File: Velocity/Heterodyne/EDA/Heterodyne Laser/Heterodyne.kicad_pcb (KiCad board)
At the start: 2 copper layers, 35.5 x 19 mm, 38 parts, among them J1 Conn_01x05, J7 Reciever, U1 SA612AD, U2 NE5532DR, U3 MAX7375AXR105, U4 MAX11613, U5 ATmega328PB-AU, Y1 8 MHz

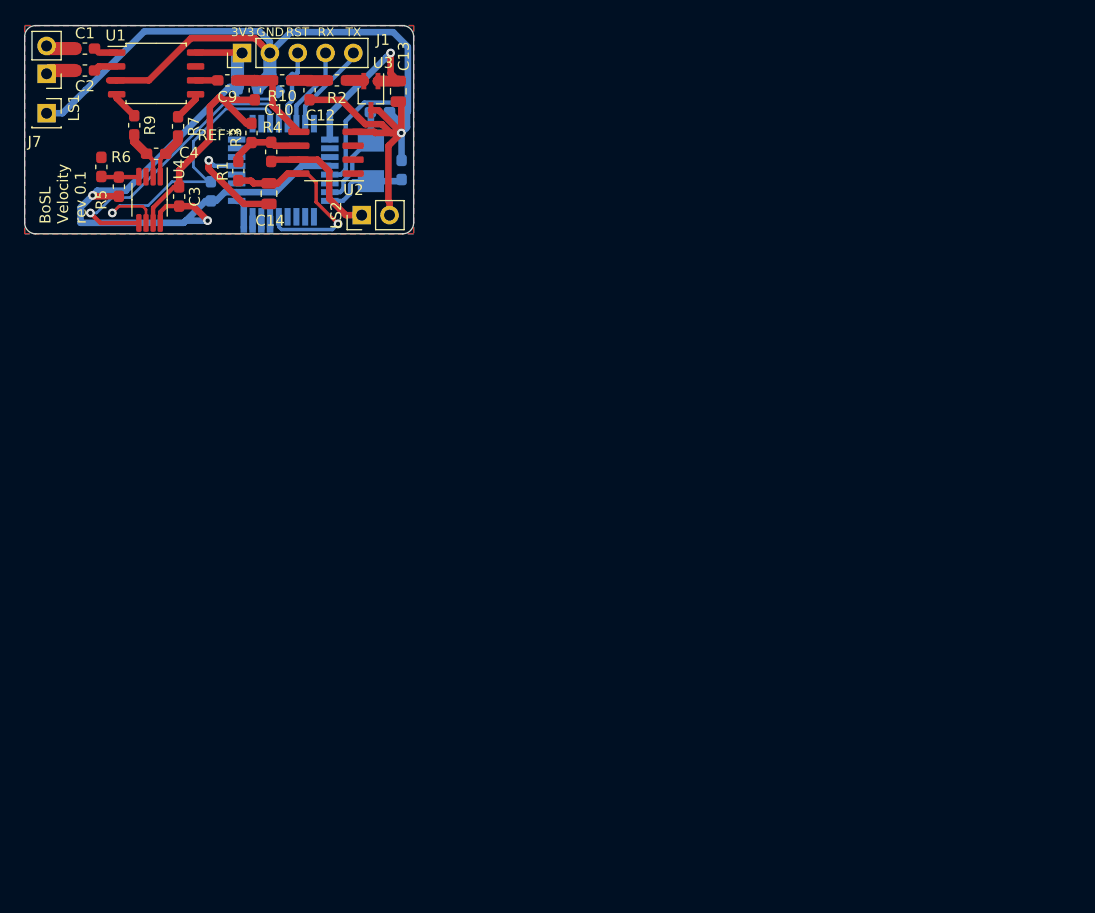
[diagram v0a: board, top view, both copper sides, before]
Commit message: daily commit
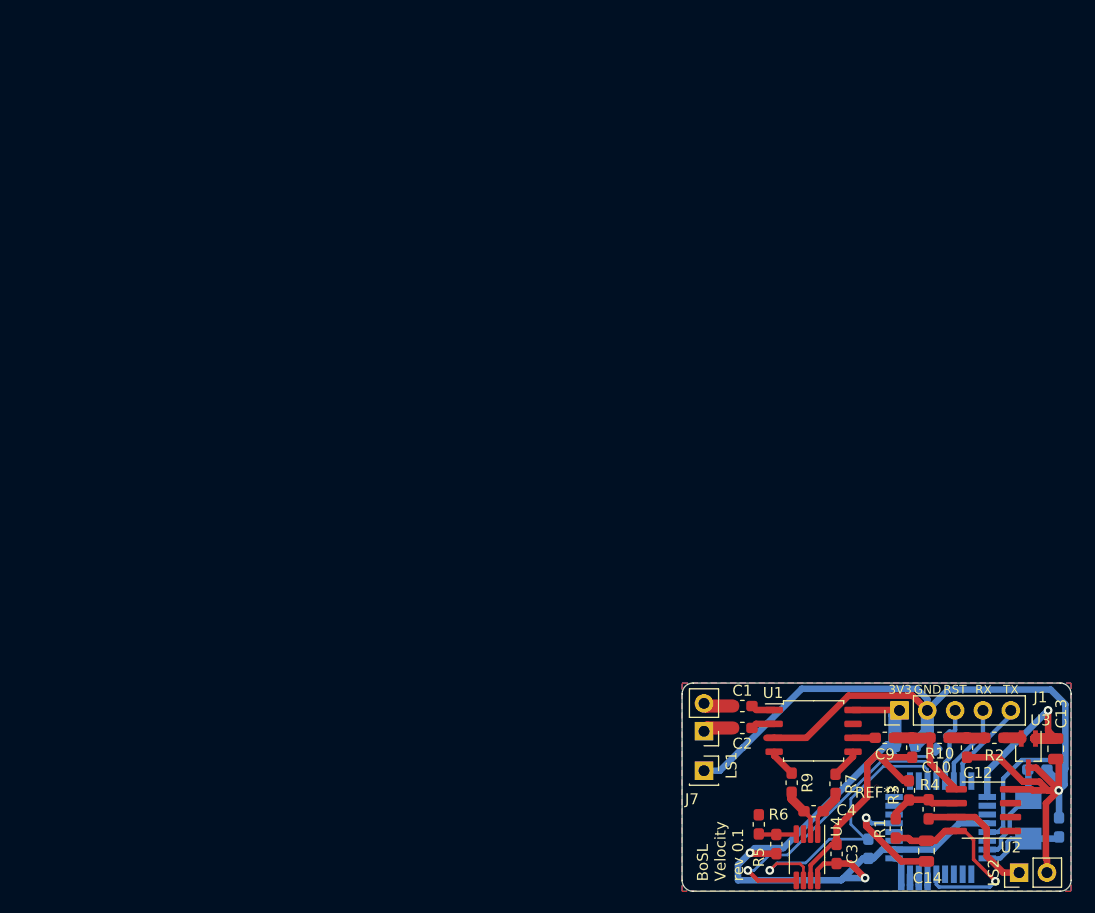
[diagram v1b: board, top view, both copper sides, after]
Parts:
- moved U4 84.9 mm to (71.4, 75.9)
- moved C1 84.9 mm to (65.5, 62.1)
- moved C10 84.9 mm to (81.0, 65.9)
- moved C12 84.9 mm to (86.0, 65.9)
- moved C14 84.9 mm to (82.3, 75.3)
- moved C4 84.9 mm to (72.0, 71.7)
- moved C5 84.9 mm to (92.4, 67.9)
- moved C6 84.9 mm to (94.4, 73.2)
- moved C9 84.9 mm to (78.5, 65.0)
- moved J1 84.9 mm to (79.8, 62.5)
- moved J7 84.9 mm to (62.0, 68.0)
- moved LS1 84.9 mm to (62.0, 64.4)
- moved LS2 84.9 mm to (90.8, 77.3)
- moved R1 84.9 mm to (79.5, 73.3)
- moved R10 84.9 mm to (83.5, 65.0)
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
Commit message: fixed merge files with master
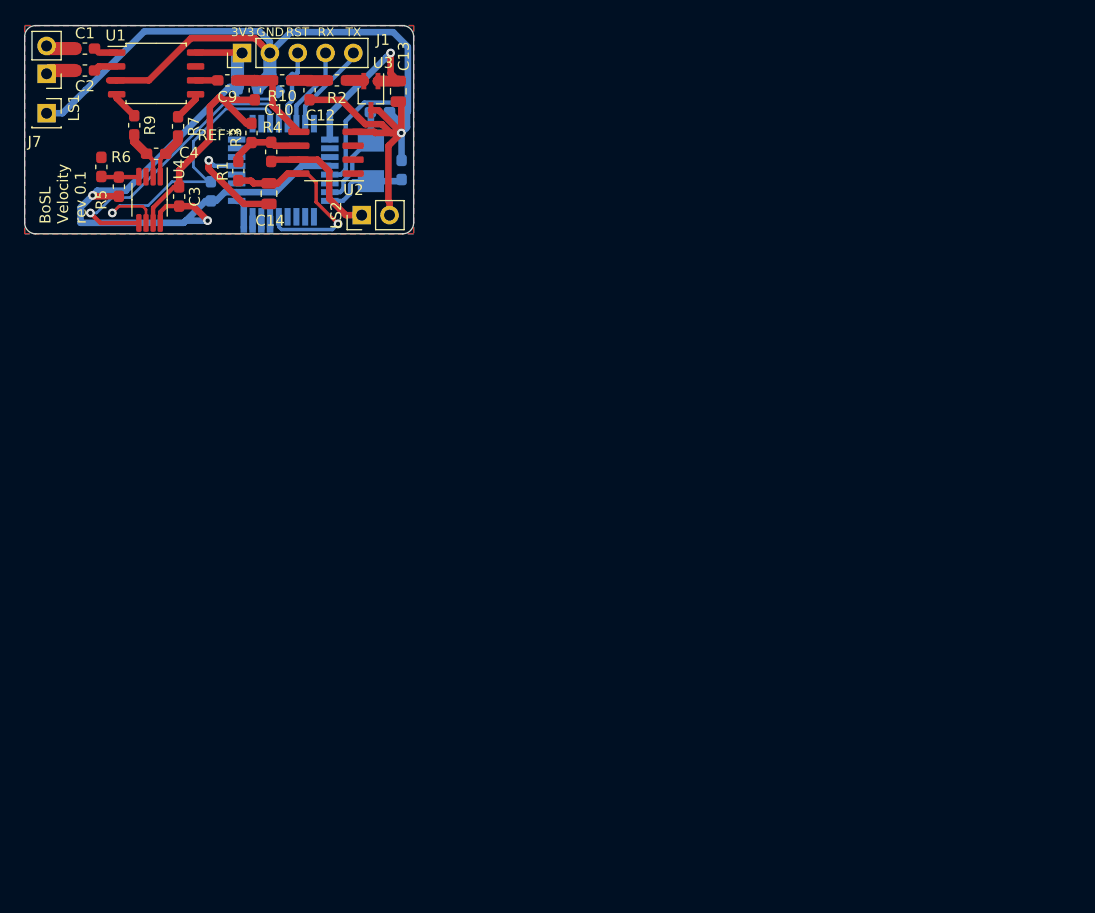
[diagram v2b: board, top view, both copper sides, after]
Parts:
- moved U4 84.9 mm to (11.4, 15.9)
- moved C1 84.9 mm to (5.50, 2.10)
- moved C10 84.9 mm to (21.0, 5.90)
- moved C12 84.9 mm to (26.0, 5.90)
- moved C14 84.9 mm to (22.3, 15.3)
- moved C4 84.9 mm to (12.0, 11.7)
- moved C5 84.9 mm to (32.4, 7.90)
- moved C6 84.9 mm to (34.4, 13.2)
- moved C9 84.9 mm to (18.5, 5.00)
- moved J1 84.9 mm to (19.8, 2.50)
- moved J7 84.9 mm to (2.00, 8.00)
- moved LS1 84.9 mm to (2.00, 4.40)
- moved LS2 84.9 mm to (30.8, 17.3)
- moved R1 84.9 mm to (19.5, 13.3)
- moved R10 84.9 mm to (23.5, 5.00)
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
